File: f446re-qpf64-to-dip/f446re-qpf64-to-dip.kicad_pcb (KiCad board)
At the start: 2 copper layers, 32 x 83 mm, 4 parts, among them J1 Conn_01x32_Pin, J2 Conn_01x32_Pin, U1 STM32F446RETx

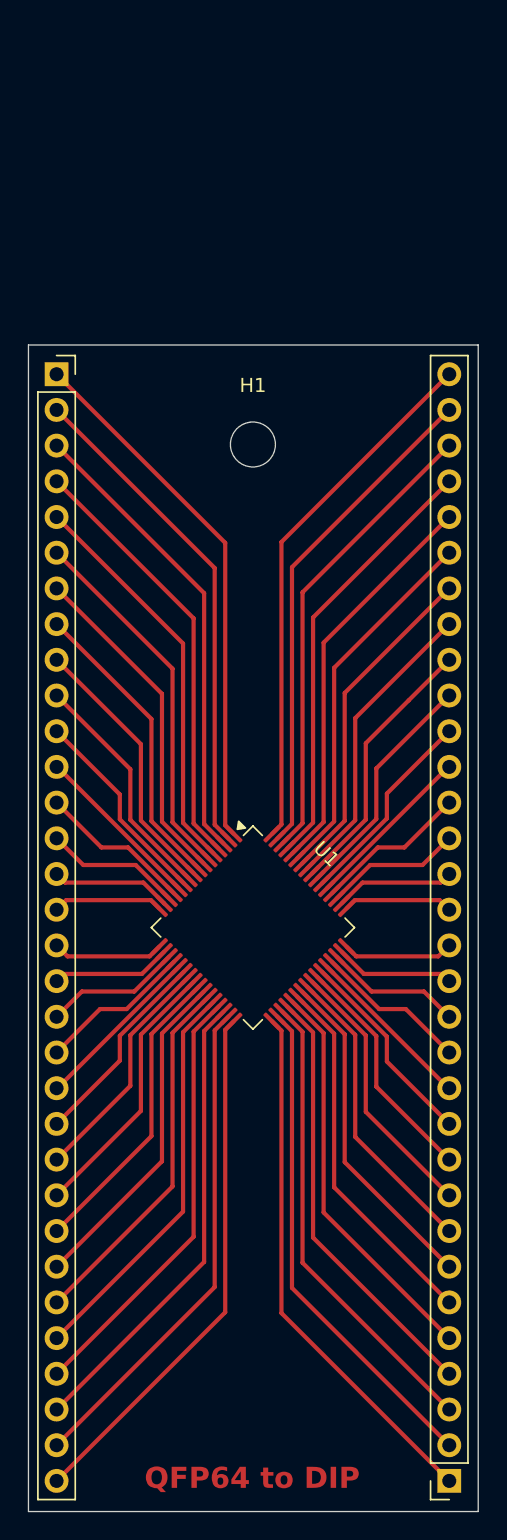
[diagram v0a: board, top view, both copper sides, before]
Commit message: change: 配線変更
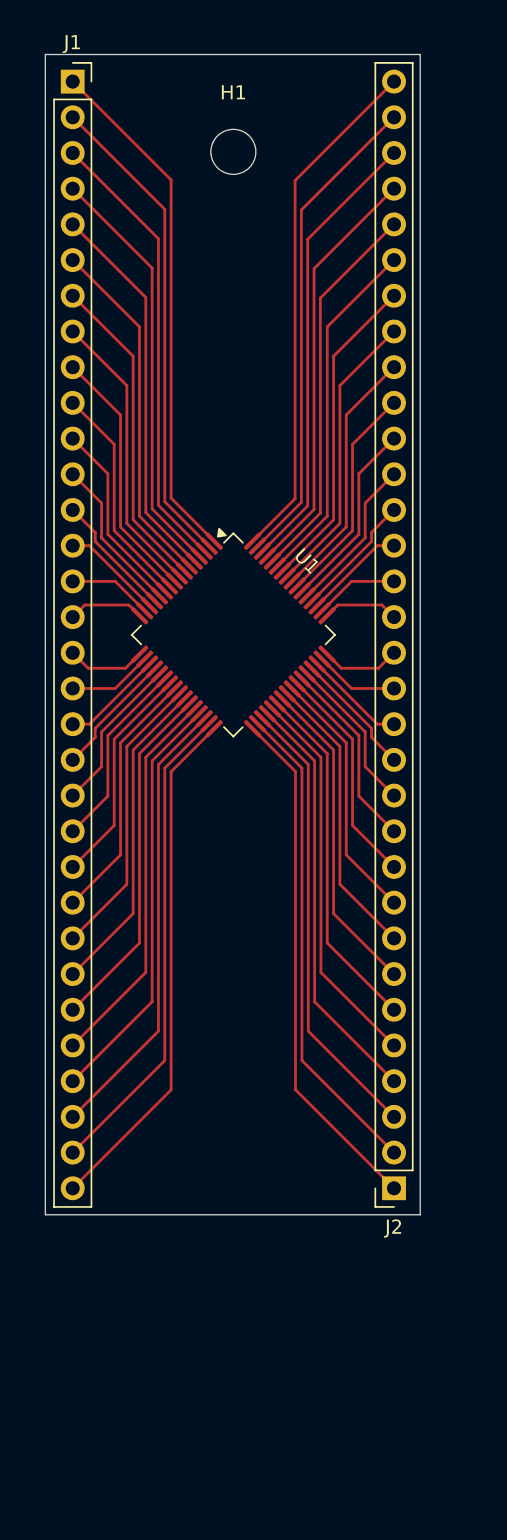
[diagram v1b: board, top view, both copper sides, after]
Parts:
- moved J2 21.2 mm to (117.0, 141.5)
- moved U1 20.9 mm to (105.6, 102.1)
- moved H1 20.9 mm to (105.6, 67.8)
- moved J1 20.9 mm to (94.2, 62.8)
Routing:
- net Net-(J1-Pin_18): track 88.2 -> 81.1 mm
- net Net-(J1-Pin_15): track 8.53 -> 5.99 mm
- net Net-(J1-Pin_14): track 9.79 -> 7.25 mm
- net Net-(J1-Pin_19): track 9.79 -> 7.25 mm
- net Net-(J2-Pin_19): track 9.79 -> 7.25 mm
- net Net-(J2-Pin_14): track 9.79 -> 7.25 mm
- net Net-(J2-Pin_18): track 8.53 -> 5.99 mm
- net Net-(J1-Pin_16): track 7.83 -> 5.44 mm
- net Net-(J2-Pin_17): track 7.83 -> 5.44 mm
- net Net-(J1-Pin_17): track 7.91 -> 5.64 mm
- net Net-(J2-Pin_16): track 7.91 -> 5.64 mm
- net Net-(J1-Pin_13): track 11.0 -> 8.88 mm
- net Net-(J1-Pin_20): track 11.0 -> 8.88 mm
- net Net-(J2-Pin_20): track 11.0 -> 8.88 mm
- net Net-(J2-Pin_13): track 11.0 -> 8.88 mm
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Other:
- board size 32 x 83 mm -> 26.7 x 82.6 mm
- board text removed: "QFP64 to DIP"
